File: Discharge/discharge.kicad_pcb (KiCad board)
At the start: 2 copper layers, 51.2 x 24.2 mm, 5 parts, among them J1 HV_Conn_IN, J2 LV_Conn_IN

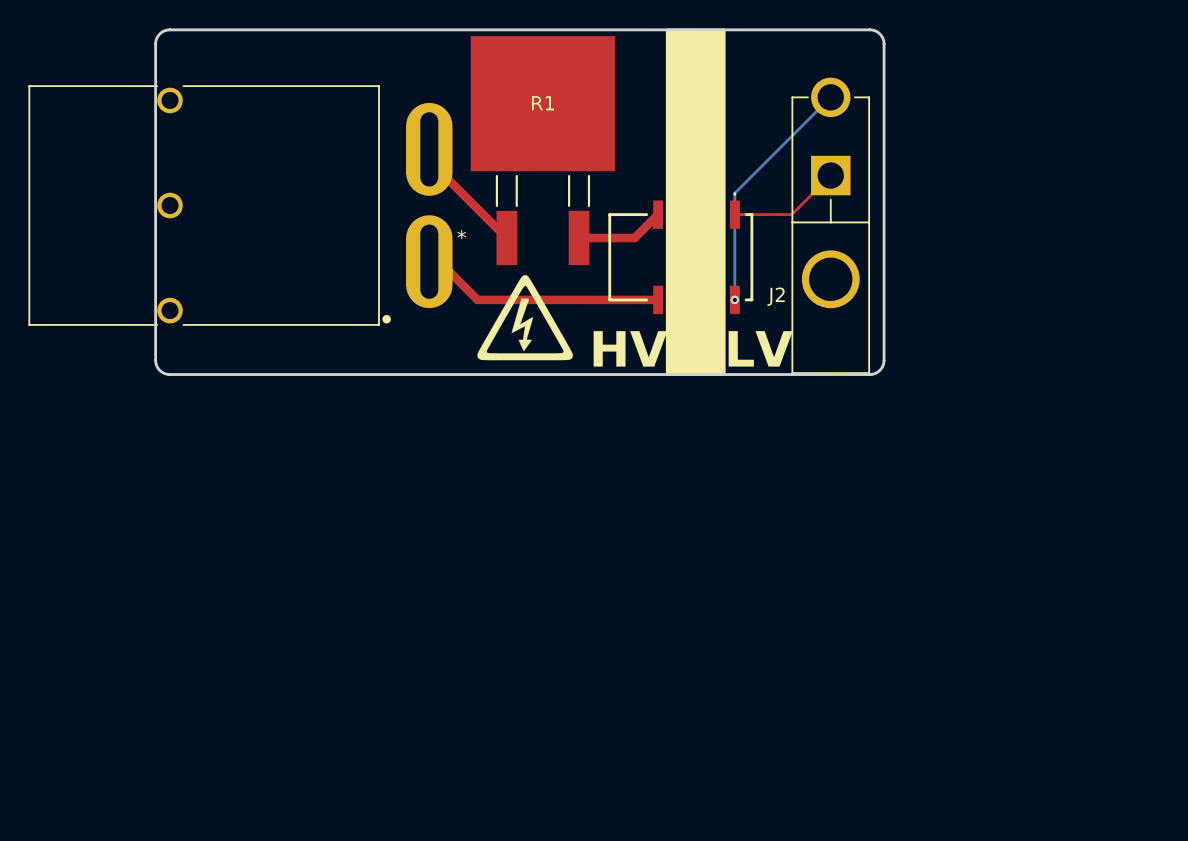
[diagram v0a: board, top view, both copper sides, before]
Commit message: Add files via upload
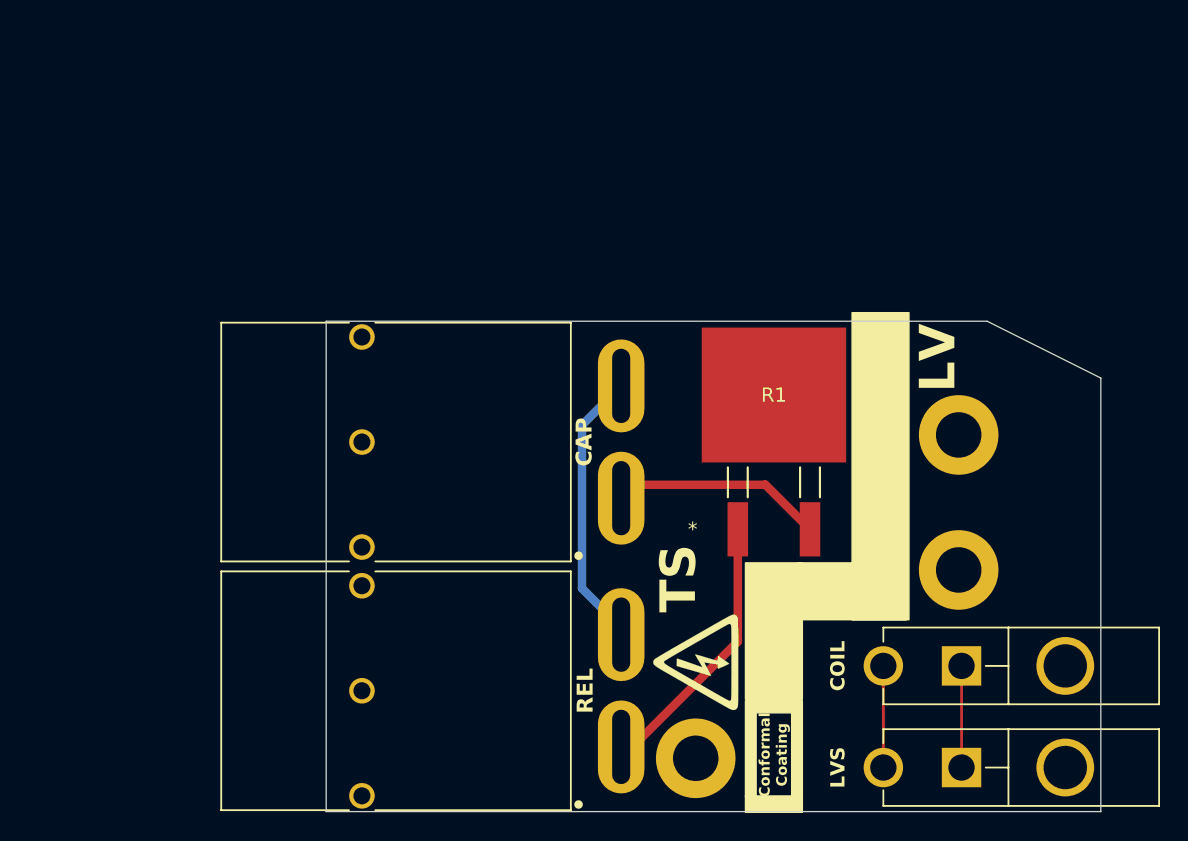
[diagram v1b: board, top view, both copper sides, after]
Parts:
- removed IMB06IGR1: S1, customFootprints:IMB03IGR
- removed J1: HV_Conn_IN, customFootprints:APP_ASMPR45-1X2-RK
- removed J2: LV_Conn_IN, molexMiniFitJr:MFJ_2X1
- added CAP: HV_Conn_IN, customFootprints:APP_ASMPR45-1X2-RK, F.Cu at (107.0, 108.5)
- added COIL: REL_COIL, molexMiniFitJr:MFJ_2X1, F.Cu at (149.2, 124.2)
- added G***: LOGO, customFootprints:electric-shock-symbol, B.Cu at (130.5, 124.0)
- added LVS: LV_Conn_IN, molexMiniFitJr:MFJ_2X1, F.Cu at (149.2, 131.4)
- added REF**: MountingHole_3.2mm_M3_DIN965_Pad, MountingHole:MountingHole_3.2mm_M3_DIN965_Pad, F.Cu at (149.0, 117.5)
- added REF**: MountingHole_3.2mm_M3_DIN965_Pad, MountingHole:MountingHole_3.2mm_M3_DIN965_Pad, F.Cu at (130.5, 130.8)
- added REF**: MountingHole_3.2mm_M3_DIN965_Pad, MountingHole:MountingHole_3.2mm_M3_DIN965_Pad, F.Cu at (149.0, 108.0)
- added REL: REL_SW, customFootprints:APP_ASMPR45-1X2-RK, F.Cu at (107.0, 126.0)
- moved G*** 27.1 mm to (130.5, 124.0), turned to 90 degrees
- moved R1 26.2 mm to (136.0, 105.2)
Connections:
- R1 pad 1: INV - -> Net-(J3-Pin_1)
- R1 pad 2: Net-(IMB06IGR1-Pad3) -> INV +
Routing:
- net Net-(J3-Pin_1): track 0.00 -> 19.2 mm
- net INV -: track 8.68 -> 19.3 mm
- net GND: track 17.0 -> 7.15 mm, vias 1 -> 0
- net Net-(IMB06IGR1-Pad3): track 6.24 -> 0.00 mm
- net INV +: track 16.8 -> 15.0 mm
- net +12V: track 7.89 -> 7.15 mm
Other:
- board size 51.2 x 24.2 mm -> 54.5 x 34.5 mm
- board text added: "Conformal Coating"
- board text added: "TS"
- board text removed: "HV"
